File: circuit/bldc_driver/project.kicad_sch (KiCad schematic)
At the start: 0 parts

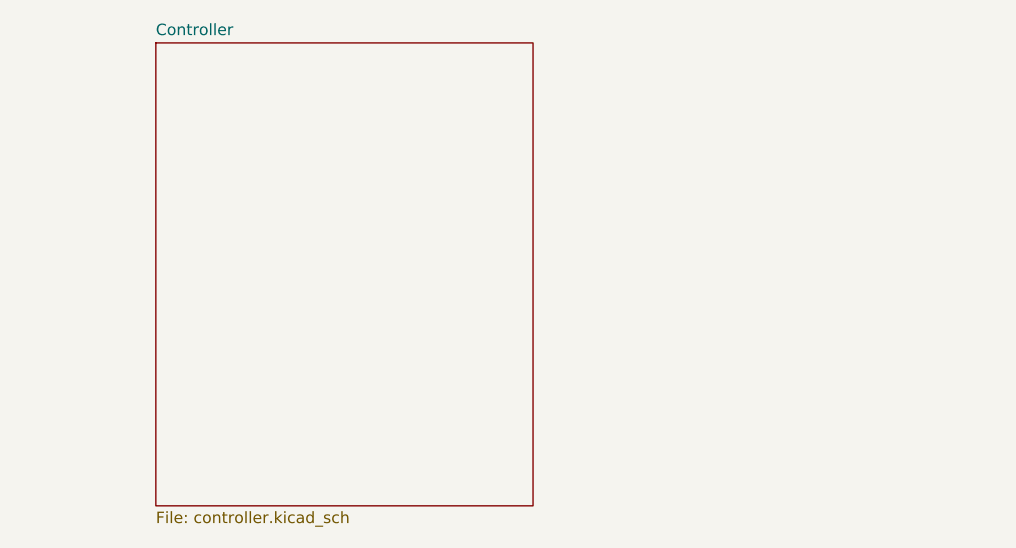
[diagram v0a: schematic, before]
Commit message: Add BLDC driver circuit.
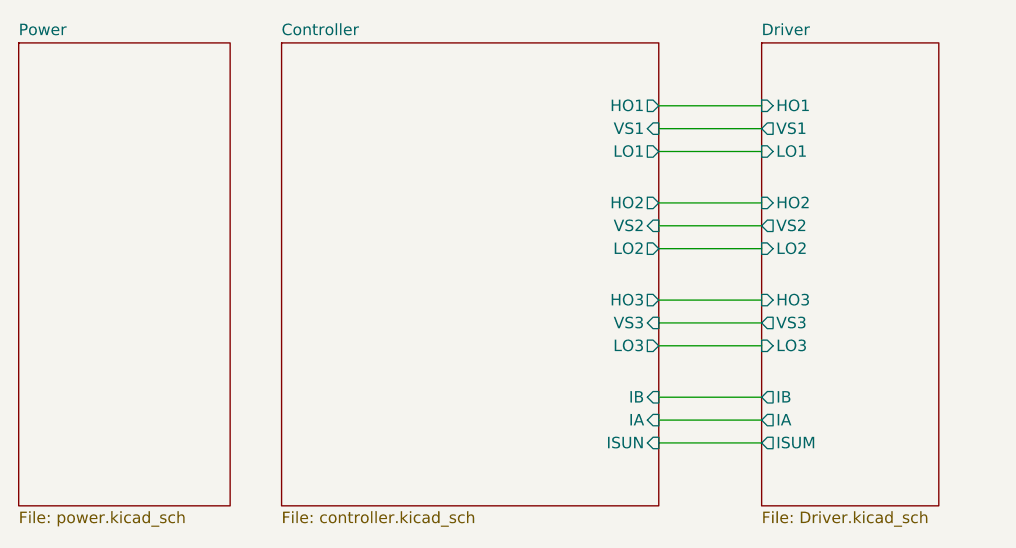
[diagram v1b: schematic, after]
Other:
- added sheet Driver (Driver.kicad_sch)
- added sheet Power (power.kicad_sch)
- sheet Controller ports: added HO1, HO2, HO3, IA, IB, ISUN, LO1, LO2, LO3, VS1, VS2, VS3; removed none
- title: BLDC Driver -> BLDC Driver 6-Step
